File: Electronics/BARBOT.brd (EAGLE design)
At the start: 80 x 100 mm, 59 parts, among them IC1 MEGA8-P, Q1 IRLR024, Q10 A03400, Q11 A03400, Q12 A03400, Q2 16MHZ

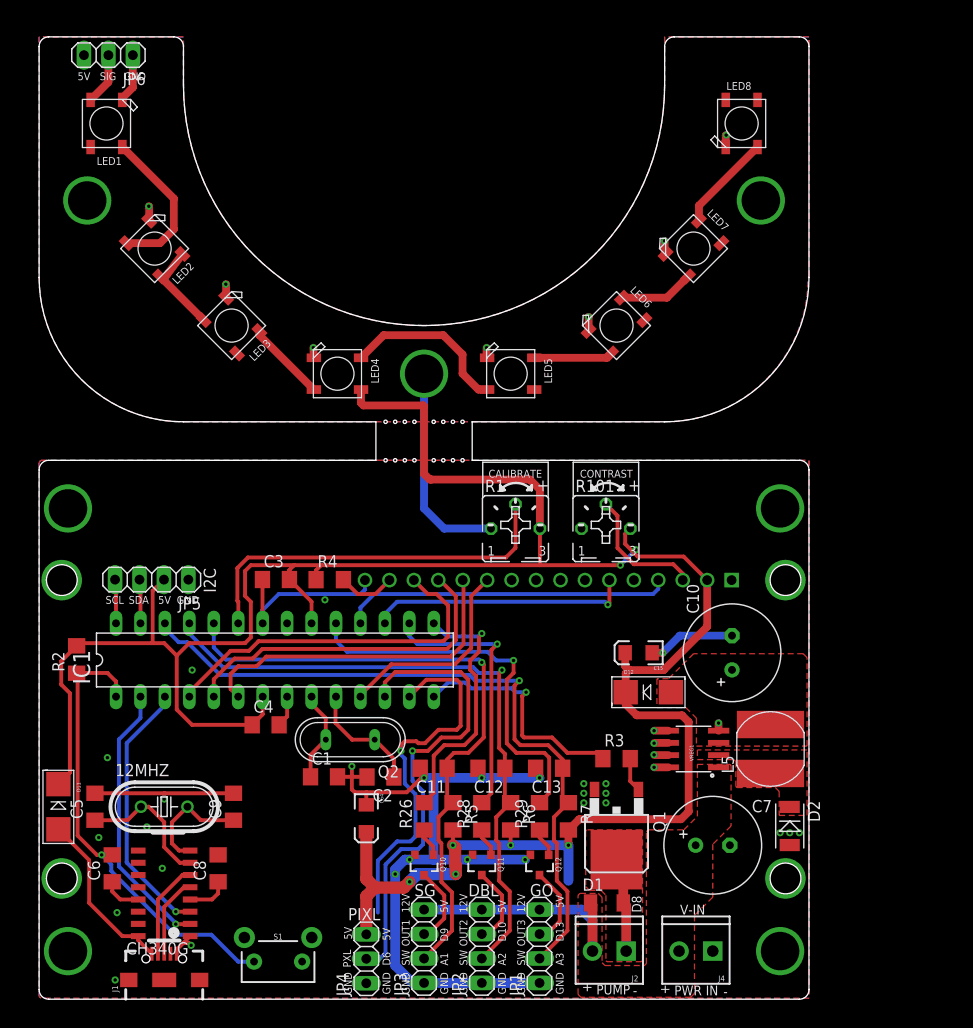
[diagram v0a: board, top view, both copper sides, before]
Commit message: CAD
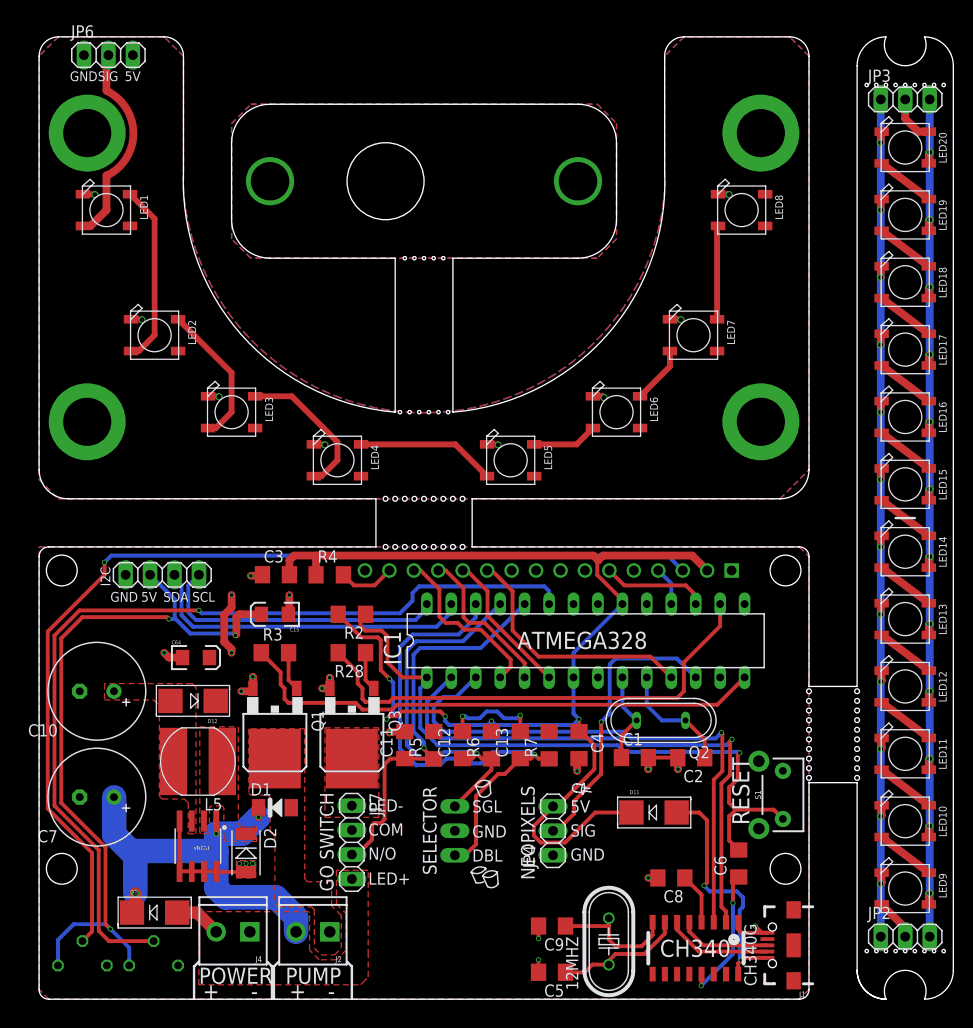
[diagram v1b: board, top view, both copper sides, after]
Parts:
- removed Q10, Q11, Q12: A03400, SparkFun-DiscreteSemi:SOT23-3
- removed R26, R29: 10R, rcl:R1206@1
- added D3: MBRA210LT3, microbuilder:SMADIODE
- added JP7: (no value), pinhead:1X04
- added LED10, LED11, LED12, LED13, LED14, LED15, LED16, LED17, LED18, LED19, LED20, LED9: WS2812B5050, adafruit:WS2812B
- added Q3: IRLR024, Cohesion_parts:D-PAK_TO252AA
- D1: value 1N4148WS-SOD323 -> M4
- JP1, JP2, JP3: device pinhead:1X04 -> pinhead:1X03
- S1: value MOMENTARY-SWITCH-SPST-PTH-RIGHT-ANGLE-KIT -> (none)
- moved JP3 101.2 mm to (90.0, 93.5), turned to 0 degrees
- moved R101 70.9 mm to (4.50, 3.50), flipped to the bottom
- moved C10 66.1 mm to (6.00, 32.0), turned to 180 degrees
- moved J1 65.5 mm to (78.4, 5.60), turned to 180 degrees
- moved C6 65.1 mm to (72.7, 14.1)
- moved C7 64.2 mm to (6.00, 21.0), turned to 180 degrees
- moved D11 61.9 mm to (63.9, 19.4), turned to 0 degrees
- moved L5 59.5 mm to (16.5, 24.7), turned to 90 degrees
- moved R1 58.9 mm to (11.9, 3.50), flipped to the bottom
- moved D2 56.6 mm to (21.5, 15.2)
- moved U$2 55.5 mm to (68.2, 5.30), turned to 180 degrees
- moved S1 55.2 mm to (77.3, 21.2), turned to 90 degrees
- moved VREG1 52.5 mm to (16.5, 15.9), turned to 180 degrees
- moved C5 50.5 mm to (53.3, 2.80), turned to 180 degrees
- moved 12MHZ 48.3 mm to (59.2, 6.00), turned to 90 degrees
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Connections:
- net D10_MSFT3 renamed D10_MSFT_GOSWITCH
- net N$17 renamed LINK2
- net N$18 renamed LINK3
- net N$19 renamed LINK4
- net N$20 renamed LINK5
- net N$21 renamed LINK6
- net N$22 renamed LINK7
- net N$23 renamed LINK8
- net N$27 renamed LINK1
- removed net A2_SW2: C12.1, IC1.25, JP2.2, R6.1
- removed net A3_SW3: C13.1, IC1.26, JP1.2, R7.1
- removed net D10OUT_SW2: JP2.3, Q11.3
- removed net D13OUT_SW3: JP1.3, Q12.3
- removed net D13_MSFT4: IC1.19, R29.2
- removed net D9OUT_SW1: JP3.3, Q10.3
- removed net N$81: Q10.1, R26.1
- removed net N$83: Q12.1, R29.1
- new net 5V1: JP2.3, JP3.3, LED10.1-VDD, LED11.1-VDD, LED12.1-VDD, LED13.1-VDD, LED14.1-VDD, LED15.1-VDD, LED16.1-VDD, LED17.1-VDD, LED18.1-VDD, LED19.1-VDD, LED20.1-VDD, LED9.1-VDD
- new net A2_SW_SINGLE: C12.1, IC1.25, JP1.1, R6.1
- new net A3_SW_DOUBLE: C13.1, IC1.26, JP1.3, R7.1
- new net D10OUT_GOSWITCH: JP7.1, Q3.4
- new net D13: IC1.19
- new net GND1: JP2.1, JP3.1, LED10.3-GND, LED11.3-GND, LED12.3-GND, LED13.3-GND, LED14.3-GND, LED15.3-GND, LED16.3-GND, LED17.3-GND, LED18.3-GND, LED19.3-GND, LED20.3-GND, LED9.3-GND
- new net LINK10: LED10.4-DIN, LED9.2-DOUT
- new net LINK11: LED10.2-DOUT, LED11.4-DIN
- new net LINK12: LED11.2-DOUT, LED12.4-DIN
- new net LINK13: LED12.2-DOUT, LED13.4-DIN
- new net LINK14: LED13.2-DOUT, LED14.4-DIN
- new net LINK15: LED14.2-DOUT, LED15.4-DIN
- new net LINK16: LED15.2-DOUT, LED16.4-DIN
- new net LINK9: JP2.2, LED9.4-DIN
- new net N$17: LED18.2-DOUT, LED19.4-DIN
- new net N$18: LED19.2-DOUT, LED20.4-DIN
- new net N$4: D3.A, J4.2
- new net N$6: JP3.2, LED20.2-DOUT
- new net N$7: LED16.2-DOUT, LED17.4-DIN
- new net N$8: LED17.2-DOUT, LED18.4-DIN
- net 24V: now also D3.C, JP7.4; no longer J4.2, JP1.4, JP2.4, JP3.4
- net A1_SW1: now also JP7.3; no longer JP3.2
- net D9_MSFT2: no longer R26.2
- net GND: now also JP1.2, JP7.2, Q3.3; no longer JP1.1, JP2.1, JP3.1, Q10.2, Q11.2, Q12.2
- net N$82: now also Q3.1; no longer Q11.1
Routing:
- net GND: track 173.2 -> 66.8 mm, vias 43 -> 30
- net 5V1: track 0.00 -> 101.2 mm, vias 0 -> 12
- net GND1: track 0.00 -> 101.2 mm, vias 0 -> 12
- net CONTRAST: track 13.6 -> 105.1 mm, vias 0 -> 1
- net A3_SW3: track 75.1 -> 0.00 mm, vias 1 -> 0
- net A2_SW2: track 68.4 -> 0.00 mm, vias 1 -> 0
- net A0_CALIBRATE: track 40.1 -> 94.5 mm, vias 0 -> 1
- net A3_SW_DOUBLE: track 0.00 -> 54.2 mm, vias 0 -> 1
- net 5V: track 259.9 -> 209.4 mm, vias 7 -> 8
- net D13_MSFT4: track 40.1 -> 0.00 mm, vias 1 -> 0
- net A2_SW_SINGLE: track 0.00 -> 39.7 mm, vias 0 -> 1
- net D7: track 38.3 -> 0.00 mm, vias 1 -> 0
- net D8_MSFT1: track 24.8 -> 55.5 mm, vias 1 -> 0
- net CHRX: track 27.6 -> 58.1 mm
- net D12_RS: track 34.3 -> 4.05 mm
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- added copper zone on layer 1, net D10OUT_GOSWITCH
- added copper zone on layer 1, net PWRPANEL
- added copper zone on layer 16, net PWRPANEL
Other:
- board size 80 x 100 mm -> 95 x 100 mm
- board text added: "ATMEGA328"
- board text added: "Adjust Calibration to tune shot size to exactly 1 unit (test using single)"
- board text added: "BarRobots v1.1"
- board text added: "CH340"
- board text added: "COM"
- board text added: "GO SWITCH"
- board text added: "IN"
- board text added: "If LCD is unreadable, adjust Contrast"
- board text added: "LED+"
- board text added: "LED-"
- board text added: "N/O"
- board text added: "NEOPIXELS"
- board text added: "OUT"
- board text added: "POWER"
- board text added: "RESET"
- board text added: "SELECTOR"
- board text added: "SGL"
- board text added: "WS2812 ADDR RGB LEDS"
- board text added: "x12"
- board text removed: "A1"
- board text removed: "A2"
- board text removed: "A3"
- board text removed: "D10"
- board text removed: "D13"
- board text removed: "D6"
- board text removed: "D8"
- board text removed: "D9"
- board text removed: "GO"
- board text removed: "OUT1"
- board text removed: "OUT2"
- board text removed: "OUT3"
- board text removed: "PIXL"
- board text removed: "PWR IN"
- board text removed: "PXL"
- board text removed: "SG"
- board text removed: "SW"
- board text removed: "V-IN"
